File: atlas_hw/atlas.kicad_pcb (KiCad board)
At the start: 4 copper layers, 41.9 x 57 mm, 155 parts, among them J1 USB_C_Receptacle_USB2.0, J10 PSP_LCD, J11 UART3_EXT, J13 IO_MAIN, J2 DEBUG_STM, J3 PSP_TOUCH, J4 UPDI_DSS, J5 CELL_THERM, J6 LPM027M128B, J7 FLEX_12380-03, J8 Micro_SD_Card_Det, J9 PSP_LCD_BL, Q1 Q_NMOS_DGS, Q2 Q_NMOS_DGS, Q4 Q_NMOS_DGS, Q5 Q_NMOS_DGS, SW3 ResetSTM, U1 STM32H723VITx, U10 BQ25611D, U11 L96-M33, U13 LSF0108, U14 NPP600SNADJ, U15 TPS61073, U16 PAM2841, U2 S27KL0641DABHV023, U3 MCP1811B, U4 TLV62569DBV, U5 MX25L3233FM2I-08G, U6 LC709203F, U7 ATtiny402-SS, U8 MS5637, U9 MC6470, Y1 16M, Y4 32k

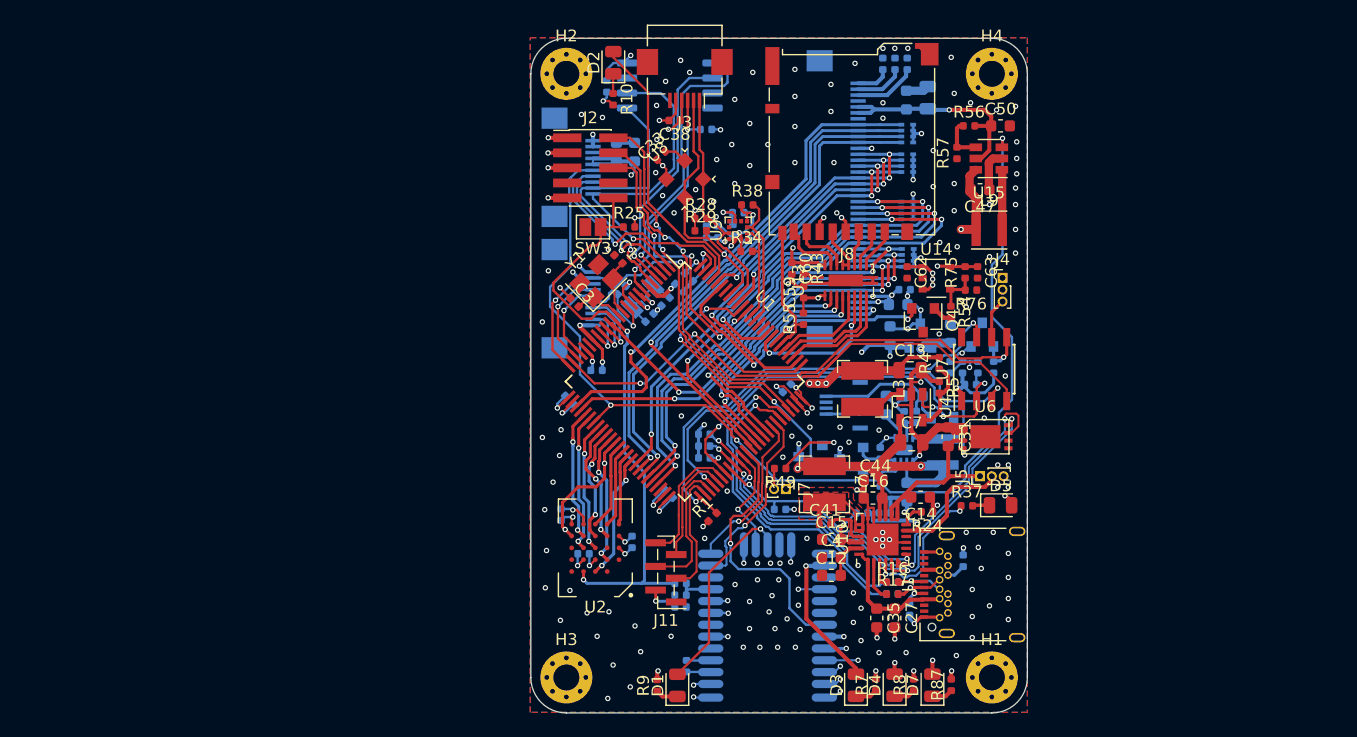
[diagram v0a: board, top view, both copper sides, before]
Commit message: atlas dev simplifcations
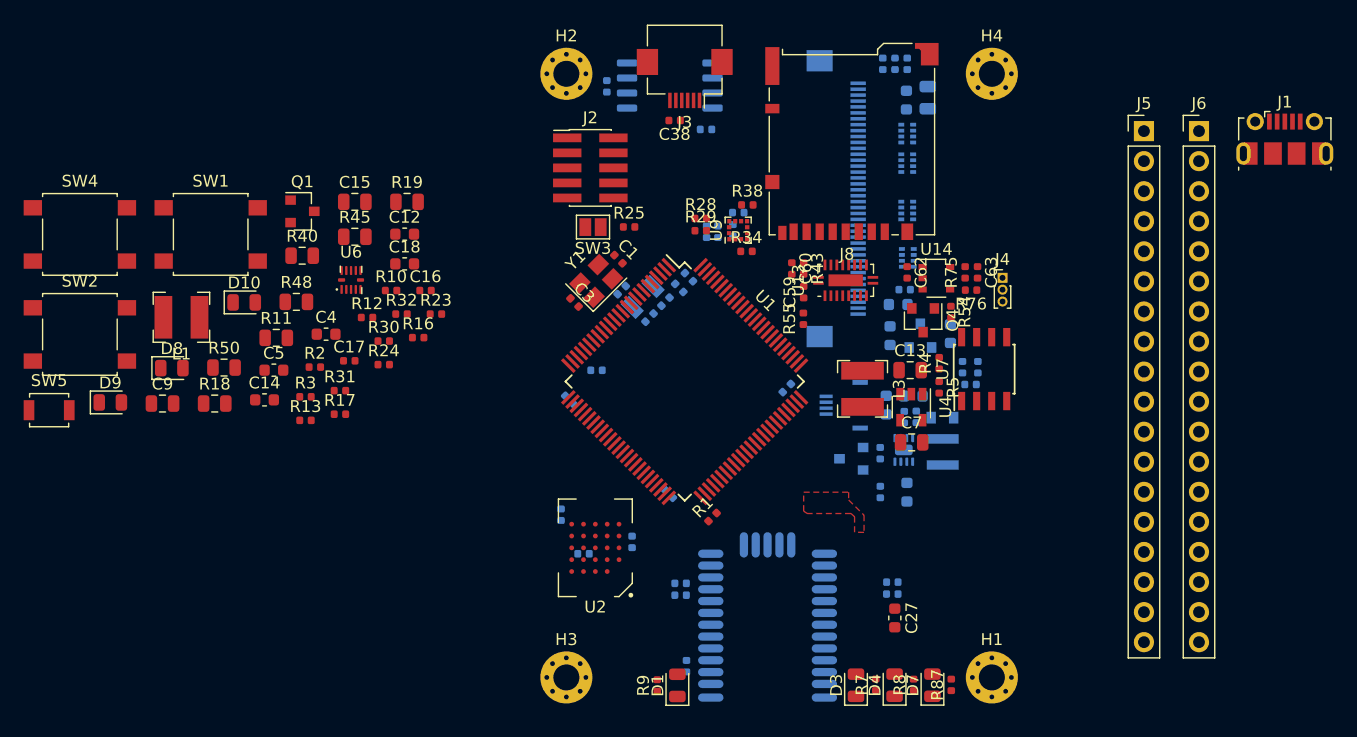
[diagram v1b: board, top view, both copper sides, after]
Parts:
- removed C31, C35, C47, C50: 1u, Capacitor_SMD:C_0603_1608Metric
- removed C33: 0.1u, Capacitor_SMD:C_0402_1005Metric
- removed C41: 47n, Capacitor_SMD:C_0402_1005Metric
- removed C44: 4.7u, Capacitor_SMD:C_0603_1608Metric
- removed D2: STM_STATUS_B, LED_SMD:LED_0805_2012Metric
- removed D5: CHARGE_STATUS, LED_SMD:LED_0805_2012Metric
- removed J11: UART3_EXT, Connector_PinHeader_1.00mm:PinHeader_1x06_P1.00mm_Vertical_SMD_Pin1Left
- removed J13: IO_MAIN, Connector_FFC-FPC:Hirose_FH12-10S-0.5SH_1x10-1MP_P0.50mm_Horizontal
- removed J7: FLEX_12380-03, Connector_PinHeader_1.00mm:PinHeader_1x02_P1.00mm_Vertical
- removed L7: 1u, Inductor_SMD:L_Bourns-SRN4018
- removed L9: L_Small, Inductor_SMD:L_Taiyo-Yuden_MD-3030
- removed Q5: Q_NMOS_DGS, Package_TO_SOT_SMD:SOT-23
- removed R33, R35: 4.7k, Resistor_SMD:R_0402_1005Metric
- removed R36, R41, R85, R86: 100k, Resistor_SMD:R_0402_1005Metric
- removed R37: 1k, Resistor_SMD:R_0402_1005Metric
- removed R49: 100, Resistor_SMD:R_0402_1005Metric
- removed R56, R57: NP, Resistor_SMD:R_0402_1005Metric
- removed U10: BQ25611D, Package_DFN_QFN:WQFN-24-1EP_4x4mm_P0.5mm_EP2.7x2.7mm
- removed U15: TPS61073, Package_TO_SOT_SMD:SOT-23-6
- removed U8: MS5637, atlas:QFN-4_3x3_Pitch2mm
- added C17: 0.1u, Capacitor_SMD:C_0402_1005Metric, F.Cu at (159.7, 112.0)
- added D10: STM_STATUS_R, LED_SMD:LED_0805_2012Metric, F.Cu at (150.8, 107.1)
- added D8: STM_STATUS_L, LED_SMD:LED_0805_2012Metric, F.Cu at (144.7, 112.6)
- added D9: STM_STATUS_0, LED_SMD:LED_0805_2012Metric, F.Cu at (139.5, 115.5)
- added L1: 2.2u, Inductor_SMD:L_Bourns-SRN4018, F.Cu at (145.5, 108.3)
- added R11: 1k, Resistor_SMD:R_0805_2012Metric, F.Cu at (153.5, 110.1)
- added R18: 1k, Resistor_SMD:R_0805_2012Metric, F.Cu at (148.3, 115.6)
- added R19: 1k, Resistor_SMD:R_0805_2012Metric, F.Cu at (164.6, 98.6)
- added R2: 100k, Resistor_SMD:R_0402_1005Metric, F.Cu at (156.8, 112.5)
- added R23: NP, Resistor_SMD:R_0402_1005Metric, F.Cu at (167.0, 108.0)
- added R3: 100k, Resistor_SMD:R_0402_1005Metric, F.Cu at (156.0, 115.0)
- added R30: NP, Resistor_SMD:R_0402_1005Metric, F.Cu at (162.6, 110.3)
- added R40: 100k, Resistor_SMD:R_0805_2012Metric, F.Cu at (155.7, 103.1)
- added R45: 100k, Resistor_SMD:R_0805_2012Metric, F.Cu at (160.2, 101.5)
- added R48: 100k, Resistor_SMD:R_0805_2012Metric, F.Cu at (155.2, 107.0)
- added R50: 100k, Resistor_SMD:R_0805_2012Metric, F.Cu at (149.1, 112.6)
- added SW1: BTN_L_EXT, Button_Switch_SMD:SW_SPST_B3S-1000, F.Cu at (148.0, 101.3)
- added SW2: BTN_0_EXT, Button_Switch_SMD:SW_SPST_B3S-1000, F.Cu at (136.9, 109.8)
- added SW4: BTN_R_EXT, Button_Switch_SMD:SW_SPST_B3S-1000, F.Cu at (136.9, 101.3)
- added SW5: BTN_PWR_EXT, Button_Switch_SMD:SW_SPST_B3U-1000P, F.Cu at (134.3, 116.2)
- C12, C14, C4: value 4.7u -> 1u
- C15: value 4.7u -> 10u; footprint Capacitor_SMD:C_0603_1608Metric -> Capacitor_SMD:C_0805_2012Metric
- C16: value 4.7u -> 0.1u; footprint Capacitor_SMD:C_0603_1608Metric -> Capacitor_SMD:C_0402_1005Metric
- C18: value 0.1u -> 10u; footprint Capacitor_SMD:C_0402_1005Metric -> Capacitor_SMD:C_0603_1608Metric; moved to F.Cu
- C5: value 0.1u -> 1u; moved to F.Cu
- C9: value 1u -> 10u; footprint Capacitor_SMD:C_0603_1608Metric -> Capacitor_SMD:C_0805_2012Metric; moved to F.Cu
- J1: value USB_C_Receptacle_USB2.0 -> USB_B_Micro; footprint Connector_USB:USB_C_Receptacle_Amphenol_12401548E4-2A -> Connector_USB:USB_Micro-B_Molex-105017-0001
- J5: value CELL_THERM -> EXP_L; footprint Connector_PinHeader_1.00mm:PinHeader_1x03_P1.00mm_Vertical -> Connector_PinHeader_2.54mm:PinHeader_1x18_P2.54mm_Vertical
- J6: value LPM027M128B -> EXP_R; footprint Connector_FFC-FPC:Hirose_FH12-10S-0.5SH_1x10-1MP_P0.50mm_Horizontal -> Connector_PinHeader_2.54mm:PinHeader_1x18_P2.54mm_Vertical; moved to F.Cu
- Q1: moved to F.Cu
- R10: value 1k -> 100k
- R12, R13: value 5.1k -> 0; moved to F.Cu
- R17, R24: value 0 -> NP
- R31, R32: value 100k -> NP; moved to F.Cu
- U6: value LC709203F -> ST1PS02; footprint atlas:WDFN-8_3x4mm_0.6mm_1.96x2.56mm -> atlas:TQFN-12_1.7x2.0mm_P0.4mm
- moved R13 56.8 mm to (156.0, 117.0), turned to 0 degrees
- moved C14 56.0 mm to (152.6, 115.3), turned to 0 degrees
- moved U6 55.2 mm to (159.9, 105.2), turned to 0 degrees
- moved J6 53.1 mm to (231.5, 92.6), turned to 0 degrees
- moved R12 52.1 mm to (161.2, 108.3), turned to 0 degrees
- moved C15 49.3 mm to (160.2, 98.6)
- moved R17 49.1 mm to (158.9, 116.5)
- moved Q1 47.7 mm to (155.8, 99.4), turned to 0 degrees
- moved R24 47.6 mm to (162.6, 112.3), turned to 0 degrees
- moved C4 46.7 mm to (157.8, 109.8)
- moved C12 46.2 mm to (164.4, 101.3)
- moved J1 45.4 mm to (238.8, 93.2), turned to 0 degrees
- moved R31 45.3 mm to (158.9, 114.5)
- moved R16 45.1 mm to (165.5, 110.0)
- moved R32 44.2 mm to (164.1, 108.0)
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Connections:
- C11 pad 1: /VCC_MCU_3V3 -> /VCC_3V3
- C12 pad 1: GND -> /VCAP2_STM
- C12 pad 2: Net-(C12-Pad2) -> GND
- C13 pad 1: /VCC_MCU_3V3 -> /VCC_3V3
- C14 pad 1: GND -> /VCAP2_STM
- C14 pad 2: /CELL_POS -> GND
- C15 pad 1: GND -> /VCC_CORE
- C15 pad 2: Net-(C15-Pad2) -> GND
- C16 pad 1: GND -> /VCAP2
- C16 pad 2: /VCC_SYS -> GND
- C18 pad 1: /VCC_MCU_3V3 -> /USB_PORT_VBUS
- C2 pad 2: /VCC_MCU_3V3 -> /VCC_3V3
- C22 pad 1: /VCC_MCU_3V3 -> /VCC_3V3
- C23 pad 1: /VCC_MCU_3V3 -> /VCC_3V3
- C24 pad 1: /VCC_MCU_3V3 -> /VCC_3V3
- C25 pad 1: /VCC_MCU_3V3 -> /VCC_3V3
- C26 pad 1: /VCC_MCU_3V3 -> /VCC_3V3
- C32 pad 1: /VCC_MCU_3V3 -> /VCC_3V3
- C34 pad 1: /VCC_MCU_3V3 -> /VCC_3V3
- C4 pad 1: GND -> /VCAP1_STM
- C4 pad 2: Net-(C12-Pad2) -> GND
- C5 pad 1: /VCC_MCU_3V3 -> /VCAP1_STM
- C51 pad 1: /VCC_LCD_PWR -> /VCC_SYS
- C53 pad 1: /VCC_LCD_PWR -> /VCC_SYS
- C56 pad 2: /VCC_MCU_3V3 -> /VCC_3V3
- C57 pad 2: /VCC_MCU_3V3 -> /VCC_3V3
- C58 pad 2: /VCC_MCU_3V3 -> /VCC_3V3
- C9 pad 1: /VCC_MCU_3V3 -> /VCC_SYS
- D4 pad 2: /VCC_MCU_3V3 -> /VCC_3V3
- J10 pad 35: /VCC_LCD_PWR -> /VCC_SYS
- J10 pad 36: /VCC_LCD_PWR -> /VCC_SYS
- J2 pad 1: /VCC_MCU_3V3 -> /VCC_3V3
- J5 pad 1: /CELL_POS -> /USB_PORT_VBUS
- J5 pad 2: /CELL_NTC -> /VCC_SYS
- J5 pad 3: GND -> /VCC_BACKUP
- J6 pad 1: /SPI4_SCK_APP -> GND
- J6 pad 10: GND -> /PE0
- J6 pad 2: /SPI4_MOSI_APP -> /SDMMC1_CKIN_PB8
- J6 pad 3: /SPI4_OPT_LCD_NCS -> /PB7
- J6 pad 4: /OPT_LCD_COM_INV -> /PB6
- J6 pad 5: /EN_LCD_PWR -> GND
- J6 pad 6: /VCC_MCU_3V3 -> /PD7
- J6 pad 7: /VCC_MCU_3V3 -> /PD6
- J6 pad 8: /EXTMODE -> /SDMMC1_VSEL_PD1
- J8 pad 9: /SDMMC1_DET -> /SD_DET
- L3 pad 2: /VCC_MCU_3V3 -> /VCC_3V3
- Q1 pad 1: Net-(Q1-Pad1) -> /VCORE_EN
- Q1 pad 2: /T3C1_LCD_BL -> /STM_VCORE_EN
- R10 pad 1: Net-(D2-Pad1) -> /STM_VCORE_GOOD
- R10 pad 2: GND -> /VCC_MCU_3V3
- R12 pad 1: GND -> /VCAP1
- R12 pad 2: Net-(J1-PadA5) -> /VCC_CORE
- R13 pad 1: Net-(J1-PadB5) -> /VCAP2
- R13 pad 2: GND -> /VCC_CORE
- R14 pad 1: /USB_STM_D- -> /USB_STM_D+
- R14 pad 2: /USB_PORT_D- -> /USB_PORT_D+
- R15 pad 1: /USB_STM_D+ -> /USB_STM_D-
- R15 pad 2: /USB_PORT_D+ -> /USB_PORT_D-
- R16 pad 1: /USB_CHGR_D- -> /VCC_SYS
- R16 pad 2: /USB_PORT_D- -> /USB_PORT_VBUS
- R17 pad 1: /USB_CHGR_D+ -> /SDMMC1_D2
- R17 pad 2: /USB_PORT_D+ -> /SD_D2
- R24 pad 1: GND -> /SDMMC1_CMD
- R24 pad 2: Net-(R24-Pad2) -> /SD_CMD
- R25 pad 2: /VCC_MCU_3V3 -> /VCC_3V3
- R31 pad 1: Net-(C15-Pad2) -> /SDMMC1_D0
- R31 pad 2: /CELL_NTC -> /SD_D0
- R32 pad 1: /CELL_NTC -> /SDMMC1_D1
- R32 pad 2: GND -> /SD_D1
- R4 pad 2: /VCC_MCU_3V3 -> /VCC_3V3
- R55 pad 1: /SDMMC1_DET -> /SD_DET
- U1 pad 1: /SPI4_SCK_APP -> /SPI4_SCK_APP_PE2
- U1 pad 100: /VCC_MCU_3V3 -> /VCC_3V3
- U1 pad 11: /VCC_MCU_3V3 -> /VCC_3V3
- U1 pad 2: /SPI4_OPT_LCD_NCS -> /PWR_ACK_DSS
- U1 pad 21: /VCC_MCU_3V3 -> /VCC_3V3
- U1 pad 24: /~USB_DET -> /PA2
- U1 pad 27: /VCC_MCU_3V3 -> /VCC_3V3
- U1 pad 4: /SPI4_MISO_APP -> /SPI4_MISO_APP_PE5
- U1 pad 48: Net-(U1-Pad48) -> /VCAP1_STM
- U1 pad 5: /SPI4_MOSI_APP -> /SPI4_MOSI_APP_PE6
- U1 pad 50: /VCC_MCU_3V3 -> /VCC_3V3
- U1 pad 51: /PWR_ACK_DSS -> /STM_VCORE_EN_PB12
- U1 pad 52: /USART3_CTS_NCP -> /STM_VCORE_D2_PB13
- U1 pad 53: /USART3_RTS_NCP -> /STM_VCORE_D1_PB14
- U1 pad 54: /PWR_SW_DSS -> /STM_VCORE_D0_PB15
- U1 pad 55: /USART3_TX_NCP -> /STM_VCORE_GOOD_PD8
- U1 pad 56: /USART3_RX_NCP -> /PD9
- U1 pad 57: /LC709203_INT -> /MC6470_INTM
- U1 pad 58: /BQ25611_INT -> /MC6470_INTA
- U1 pad 59: /I2C4_SCL_SYSTEM -> /I2C1_SCL_SENSOR
- U1 pad 60: /I2C4_SDA_SYSTEM -> /I2C1_SDA_SENSOR
- U1 pad 61: /GPS_FORCE_ON -> /STC911_INT
- U1 pad 62: /GPS_EXTINT -> /PD15
- U1 pad 7: /STC911_INT -> /PWR_SW_DSS
- U1 pad 73: Net-(U1-Pad73) -> /VCAP2_STM
- U1 pad 75: /VCC_MCU_3V3 -> /VCC_3V3
- U1 pad 82: /SDMMC1_VSEL -> /SDMMC1_VSEL_PD1
- U1 pad 85: Net-(U1-Pad85) -> /GPS_FORCE_ON
- U1 pad 86: Net-(U1-Pad86) -> /GPS_EXTINT
- U1 pad 87: /MC6470_INTM -> /PD6
- U1 pad 88: /MC6470_INTA -> /PD7
- U1 pad 92: /I2C1_SCL_SENSOR -> /PB6
- U1 pad 93: /I2C1_SDA_SENSOR -> /PB7
- U1 pad 95: /SDMMC1_CKIN -> /SDMMC1_CKIN_PB8
- U1 pad 97: /STM_STATUS_B -> /PE0
- U1 pad 98: /OPT_LCD_COM_INV -> /PE1
- U2 pad B4: /VCC_MCU_3V3 -> /VCC_3V3
- U2 pad D1: /VCC_MCU_3V3 -> /VCC_3V3
- U2 pad E4: /VCC_MCU_3V3 -> /VCC_3V3
- U5 pad 8: /VCC_MCU_3V3 -> /VCC_3V3
- U6 pad 1: GND -> Net-(R3-Pad2)
- U6 pad 2: GND -> /VCC_SYS
- U6 pad 3: /CELL_POS -> Net-(L1-Pad1)
- U6 pad 4: /LC709203_INT -> GND
- U6 pad 5: Net-(U6-Pad5) -> /VCC_CORE
- U6 pad 7: /I2C4_SDA_SYSTEM -> /STM_VCORE_GOOD
- U6 pad 8: /I2C4_SCL_SYSTEM -> Net-(R3-Pad2)
- U7 pad 5: /~USB_DET -> /DSS_EXT
- U9 pad 3: /VCC_MCU_3V3 -> /VCC_3V3
- U9 pad 7: /VCC_MCU_3V3 -> /VCC_3V3
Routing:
- net GND: track 173.9 -> 0.00 mm, vias 197 -> 0
- net /EN_LCD_PWR: track 95.8 -> 0.00 mm, vias 3 -> 0
- net /VCC_MCU_3V3: track 95.8 -> 0.00 mm, vias 40 -> 0
- net /VCC_SYS: track 91.0 -> 0.00 mm, vias 6 -> 0
- net /VCC_BACKUP: track 81.8 -> 0.00 mm, vias 5 -> 0
- net /USB_PORT_VBUS: track 57.5 -> 0.00 mm, vias 2 -> 0
- net /SW_PWR: track 53.8 -> 0.00 mm, vias 1 -> 0
- net /DEBUG_NRESET_STM: track 50.6 -> 0.00 mm, vias 2 -> 0
- net /LTDC_G5: track 48.5 -> 0.00 mm, vias 3 -> 0
- net /LTDC_G4: track 47.5 -> 0.00 mm, vias 3 -> 0
- net /~USB_DET: track 46.5 -> 0.00 mm, vias 3 -> 0
- net /I2C4_SDA_SYSTEM: track 43.8 -> 0.00 mm, vias 4 -> 0
- net /LTDC_G6: track 43.7 -> 0.00 mm, vias 3 -> 0
- net /LTDC_HS: track 43.2 -> 0.00 mm, vias 1 -> 0
- net /LTDC_VS: track 42.9 -> 0.00 mm, vias 1 -> 0
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- removed copper zone on In1.Cu, net /VCC_MCU_3V3
- removed copper zone on B.Cu, net GND
- removed copper zone on F.Cu, net GND
- removed copper zone on In2.Cu, net GND
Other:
- board outline removed
